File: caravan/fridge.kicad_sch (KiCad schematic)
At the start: 15 parts

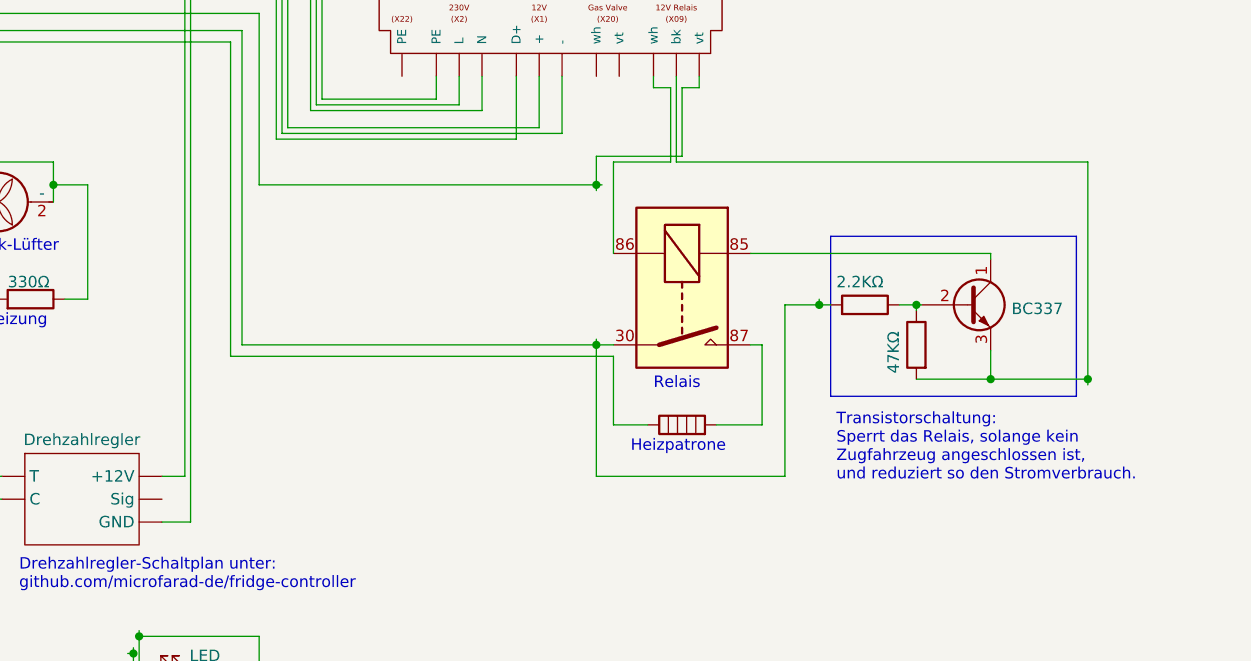
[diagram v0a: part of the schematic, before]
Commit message: Updated caravan
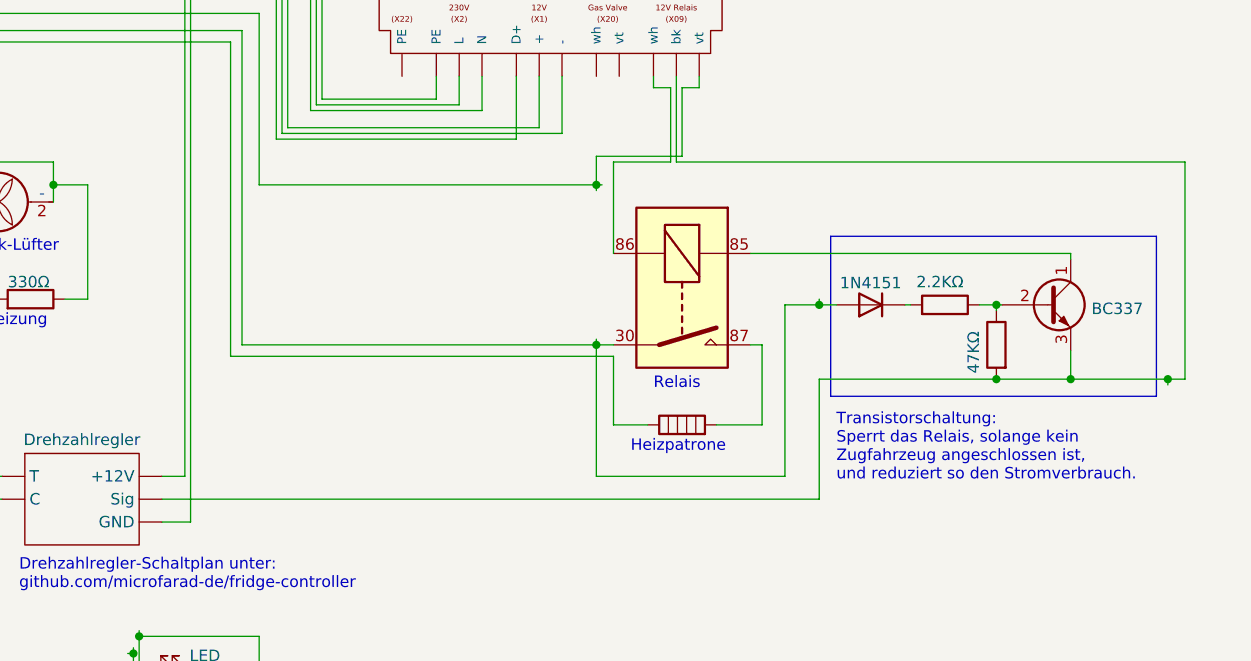
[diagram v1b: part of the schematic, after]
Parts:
- added D?: 1N4151, Diode_THT:D_DO-35_SOD27_P7.62mm_Horizontal, symbol Diode:1N4151
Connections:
- net Absorber +: now also D?.2 (A); no longer R?.2
- net at Q?.3 (E), R?.2, U?. (wh): now also U?. (T)
- new net: D?.1 (K), R?.2
- new net: U?. (T), U?. (T)
